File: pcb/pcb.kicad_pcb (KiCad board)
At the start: 2 copper layers, 161.4 x 94.6 mm, 29 parts, among them J1 Screw_Terminal_01x02, K00 Kailh Choc, K01 Kailh Choc, K02 Kailh Choc, K03 Kailh Choc, K10 Kailh Choc, K11 Kailh Choc, K12 Kailh Choc, K13 Kailh Choc, K20 Kailh Choc, K21 Kailh Choc, K22 Kailh Choc, K23 Kailh Choc, K30 Kailh Choc, K31 Kailh Choc, K32 Kailh Choc, K33 Kailh Choc, K40 Kailh Choc, K41 Kailh Choc, K42 Kailh Choc, K43 Kailh Choc, K50 Kailh Choc, K51 Kailh Choc, K52 Kailh Choc, K53 Kailh Choc, K60 Kailh Choc, K61 Kailh Choc, SW1 SW_DPST, U1 nice_nano

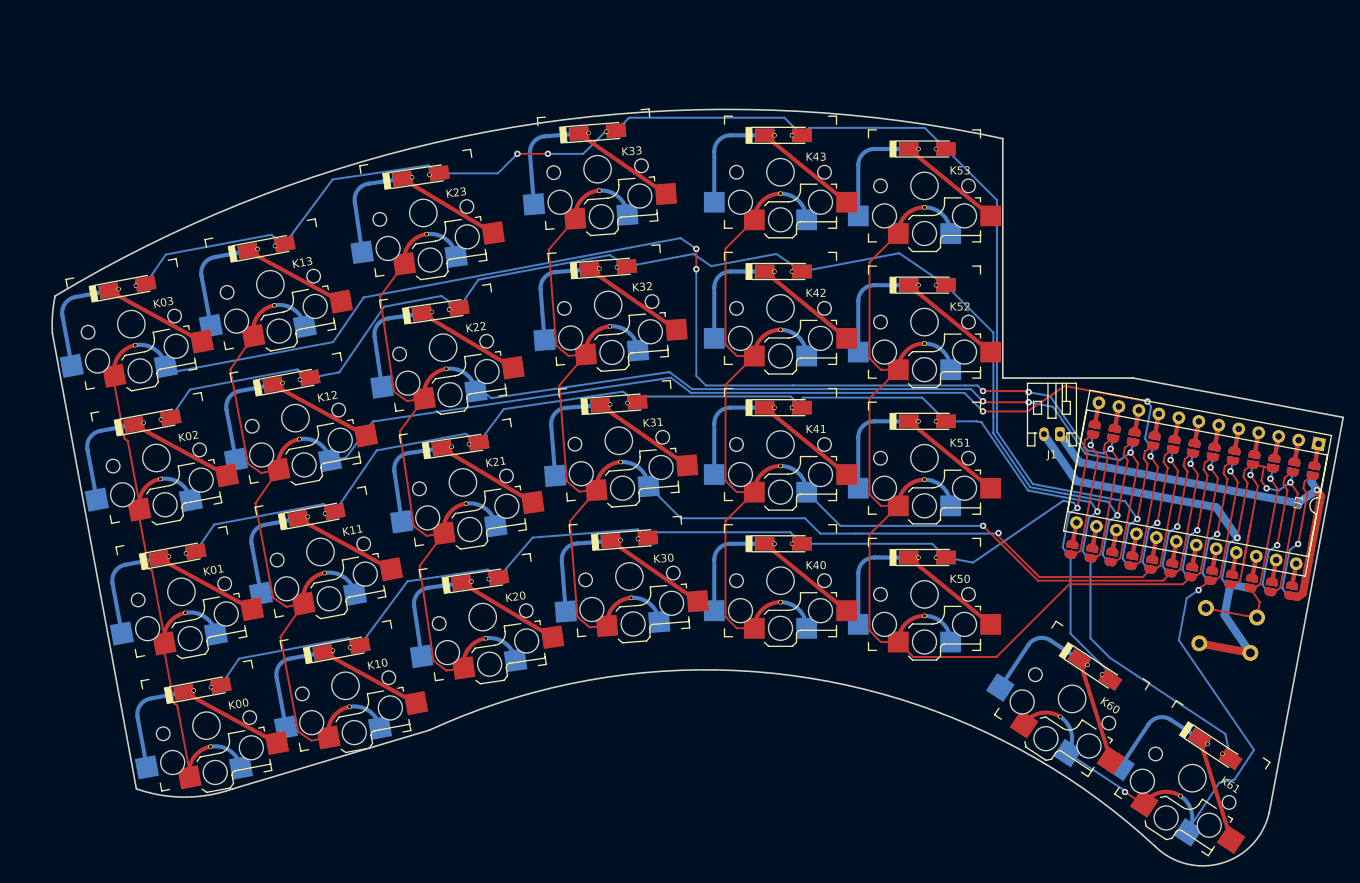
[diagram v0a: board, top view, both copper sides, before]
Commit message: refining the shape
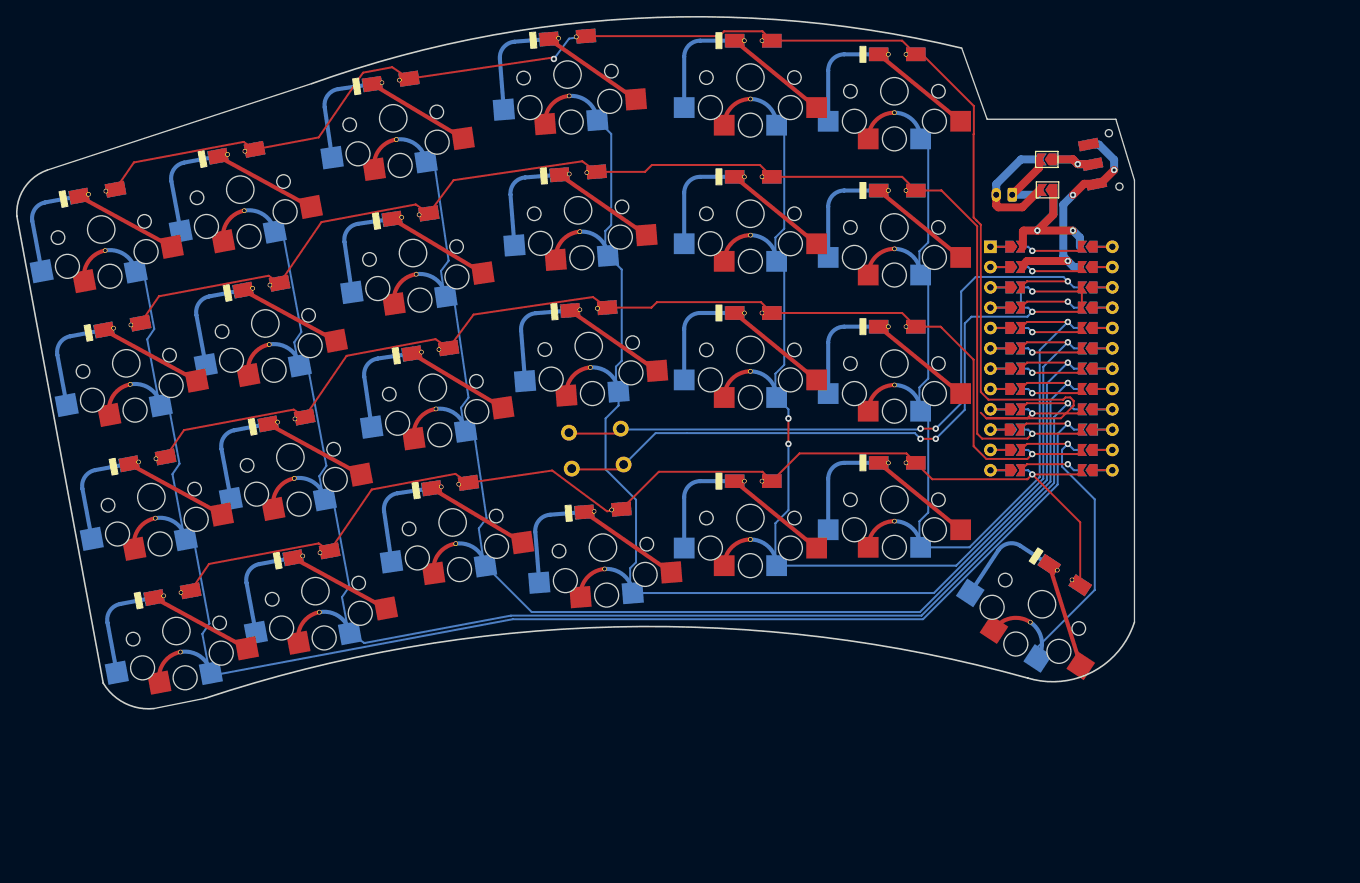
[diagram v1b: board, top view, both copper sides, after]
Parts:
- removed K61: Kailh Choc, lib:Kailh_socket_PG1350_reversible
- added JP1: SolderJumper_2_Open, Jumper:SolderJumper-2_P1.3mm_Open_TrianglePad1.0x1.5mm, F.Cu at (187.9, 64.8)
- added JP2: SolderJumper_2_Open, Jumper:SolderJumper-2_P1.3mm_Open_TrianglePad1.0x1.5mm, B.Cu at (188.0, 68.6)
- added JP3: SolderJumper_2_Open, Jumper:SolderJumper-2_P1.3mm_Open_TrianglePad1.0x1.5mm, B.Cu at (188.0, 64.8)
- added JP4: SolderJumper_2_Open, Jumper:SolderJumper-2_P1.3mm_Open_TrianglePad1.0x1.5mm, F.Cu at (188.0, 68.6)
- added SW2: SW_SPDT, lib:SW_SPDT_CK-JS102011SAQN, F.Cu at (196.3, 64.8)
- moved SW1 77.1 mm to (134.6, 98.4), turned to -175.53 degrees
- moved U1 35.1 mm to (188.4, 89.7), turned to 0 degrees
- moved J1 30.5 mm to (183.5, 69.2)
- moved K21 12.4 mm to (111.1, 93.3)
- moved K00 12.4 mm to (79.1, 123.7)
- moved K31 12.4 mm to (130.6, 88.1)
- moved K50 12.4 mm to (168.8, 107.3)
- moved K13 12.4 mm to (87.1, 68.5)
- moved K41 12.4 mm to (150.8, 88.6)
- moved K12 12.4 mm to (90.2, 85.3)
- moved K43 12.4 mm to (150.8, 54.5)
- moved K22 12.4 mm to (108.6, 76.5)
- moved K11 12.4 mm to (93.3, 102.0)
- moved K60 12.4 mm to (187.3, 120.4)
- moved K53 12.4 mm to (168.8, 56.3)
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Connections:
- J1 pad 1: Net-(U1-Pad24) -> Net-(J1-Pad1)
- J1 pad 2: GND -> Net-(J1-Pad2)
- SW1 pad 1: GND -> Net-(U1-Pad22)
- SW1 pad 2: Net-(SW1-Pad2) -> GND
- U1 pad 14: Col0 -> Col6
- U1 pad 15: Col2 -> Col0
- U1 pad 17: Col3 -> Col2
- U1 pad 18: Col4 -> Col3
- U1 pad 19: Col5 -> Col4
- U1 pad 20: Col6 -> Col5
- U1 pad 22: Net-(SW1-Pad2) -> Net-(U1-Pad22)
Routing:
- net Net-(U1-Pad22): track 0.00 -> 87.2 mm, vias 0 -> 3
- net Row1: track 181.7 -> 140.9 mm
- net Net-(U1-Pad24): track 52.0 -> 22.4 mm, vias 1 -> 2
- net GND: track 93.1 -> 122.4 mm, vias 3 -> 7
- net Col0: track 211.6 -> 183.9 mm, vias 5 -> 1
- net Col6: track 67.7 -> 40.0 mm, vias 3 -> 1
- net Net-(SW1-Pad2): track 27.1 -> 0.00 mm, vias 1 -> 0
- net Col1: track 194.2 -> 168.4 mm, vias 3 -> 1
- net Col5: track 121.7 -> 101.4 mm
- net Net-(J1-Pad2): track 0.00 -> 15.8 mm
- net unconnected-(U1-Pad21): track 21.3 -> 8.25 mm
- net Col2: track 167.6 -> 155.1 mm, vias 3 -> 1
- net Row0: track 155.7 -> 143.7 mm
- net Net-(SW2-Pad2): track 0.00 -> 10.4 mm, vias 0 -> 1
- net Net-(J1-Pad1): track 0.00 -> 9.64 mm
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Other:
- board size 161.4 x 94.6 mm -> 139.7 x 86.5 mm
- board text added: "C0,1 =10.6deg"
- board text added: "C2 = 8.36deg"
- board text added: "C3 = 4.47deg"
- board text added: "Solder jumpers on OPPOSITE side that mcu is mounted"
